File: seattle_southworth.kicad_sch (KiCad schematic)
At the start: 23 parts

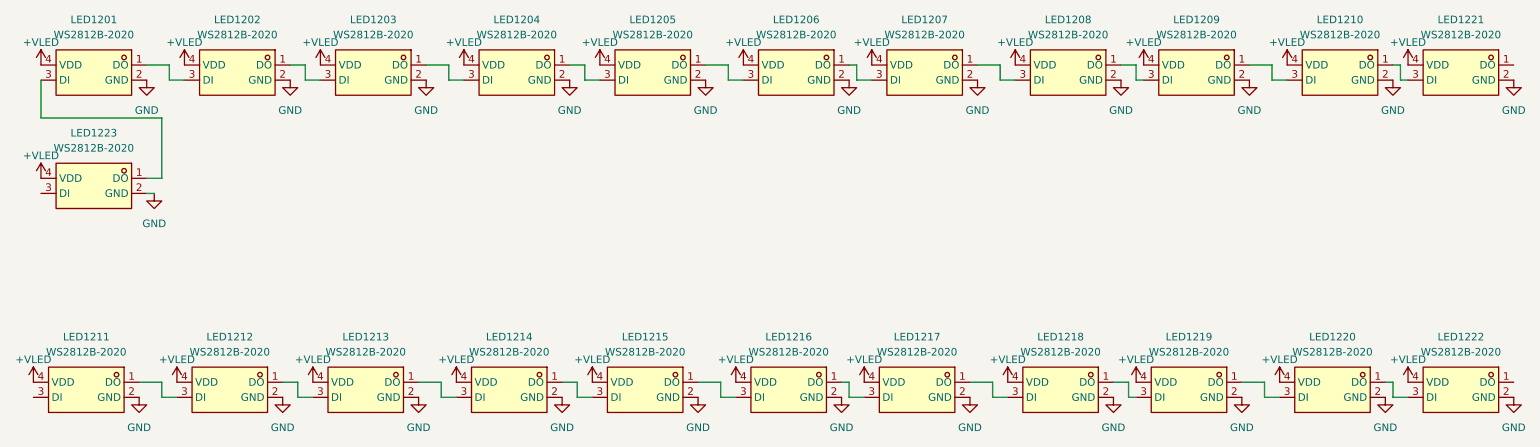
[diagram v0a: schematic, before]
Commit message: single ferry track checkpoint
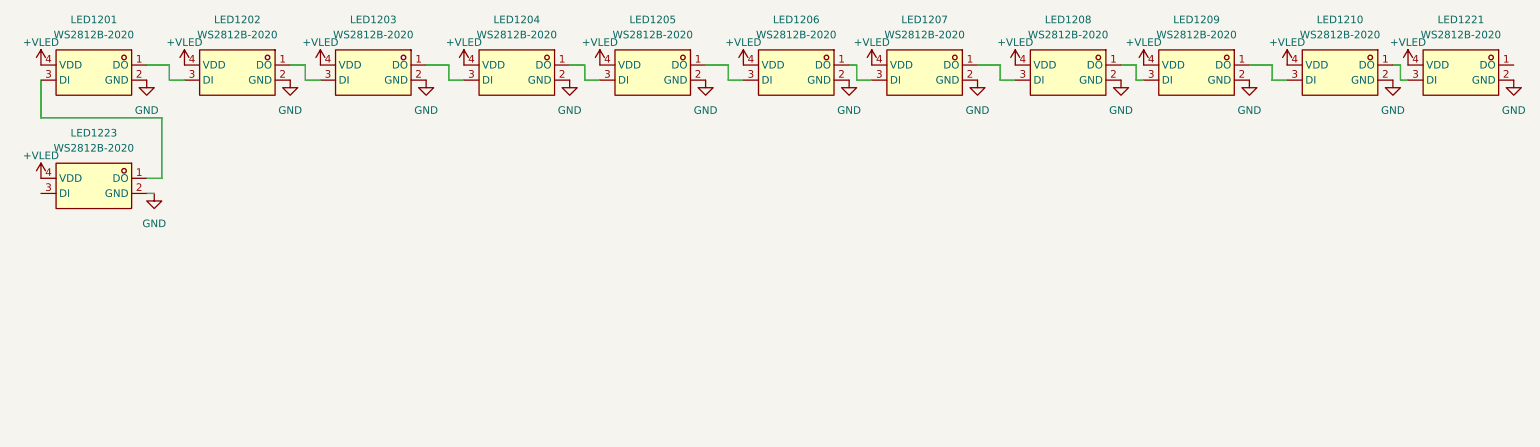
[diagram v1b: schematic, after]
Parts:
- removed LED1211, LED1212, LED1213, LED1214, LED1215, LED1216, LED1217, LED1218, LED1219, LED1220, LED1222: WS2812B-2020, EasyEDA:LED-SMD_4P-L2.0-W2.0-TL_WS2812B-2020, symbol EasyEDA:WS2812B-2020
